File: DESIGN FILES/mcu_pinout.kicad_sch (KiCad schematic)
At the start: 16 parts, among them U1 MIMXRT1064CVL5B

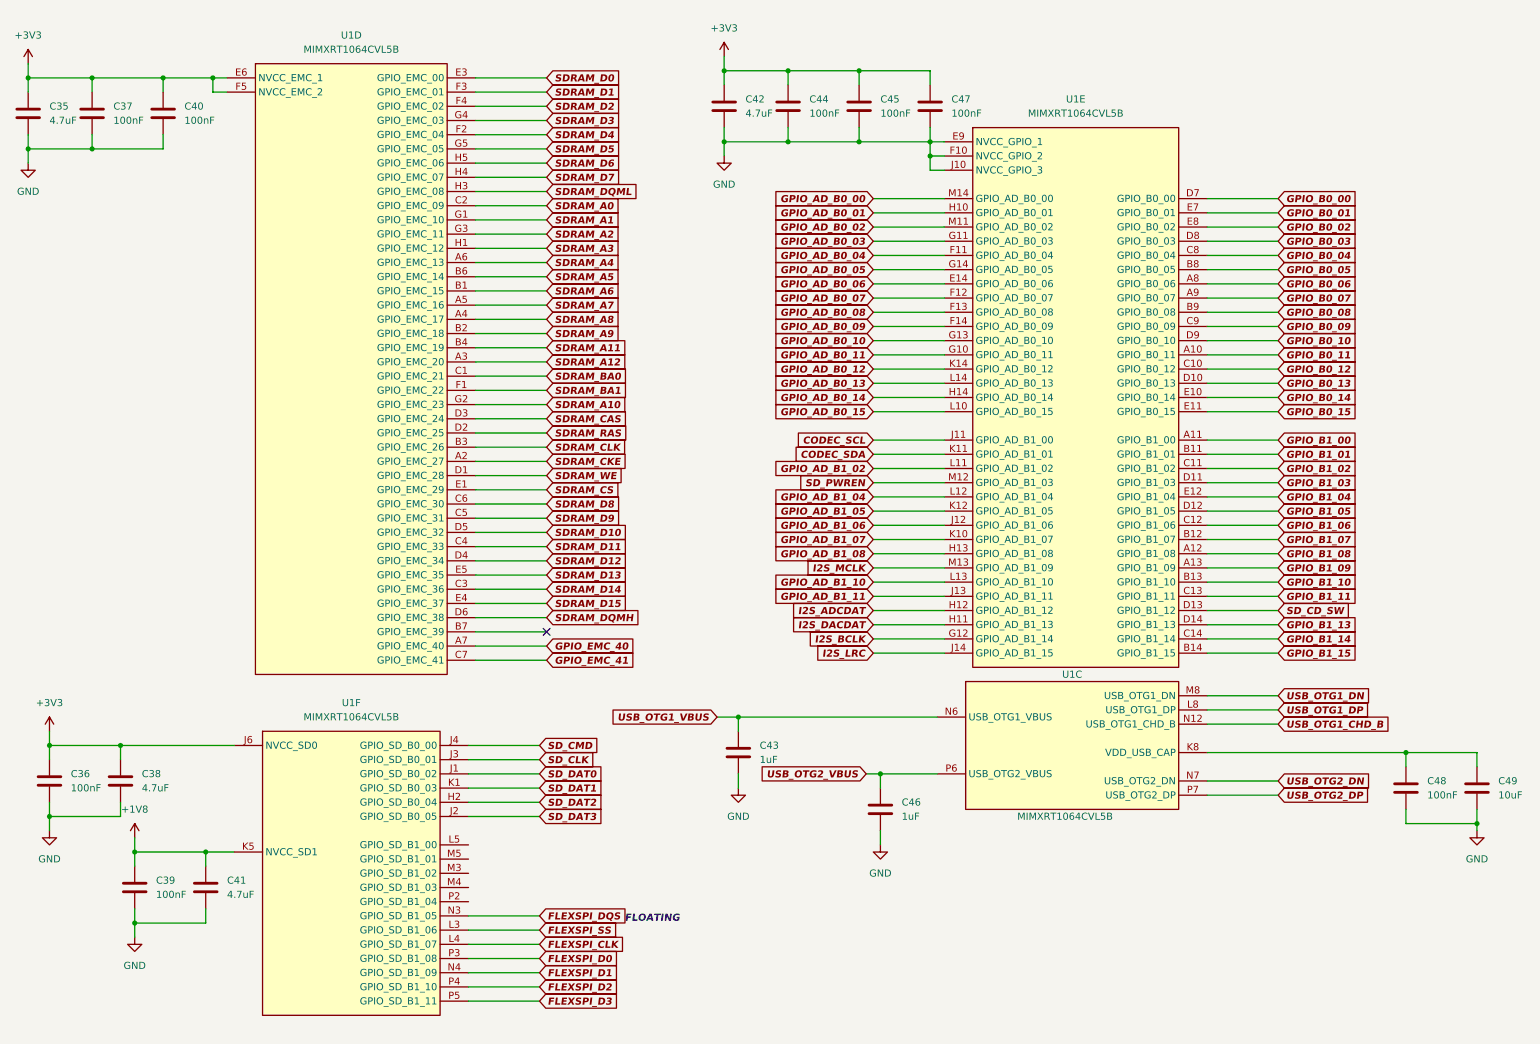
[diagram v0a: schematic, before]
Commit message: Refactoring schematic
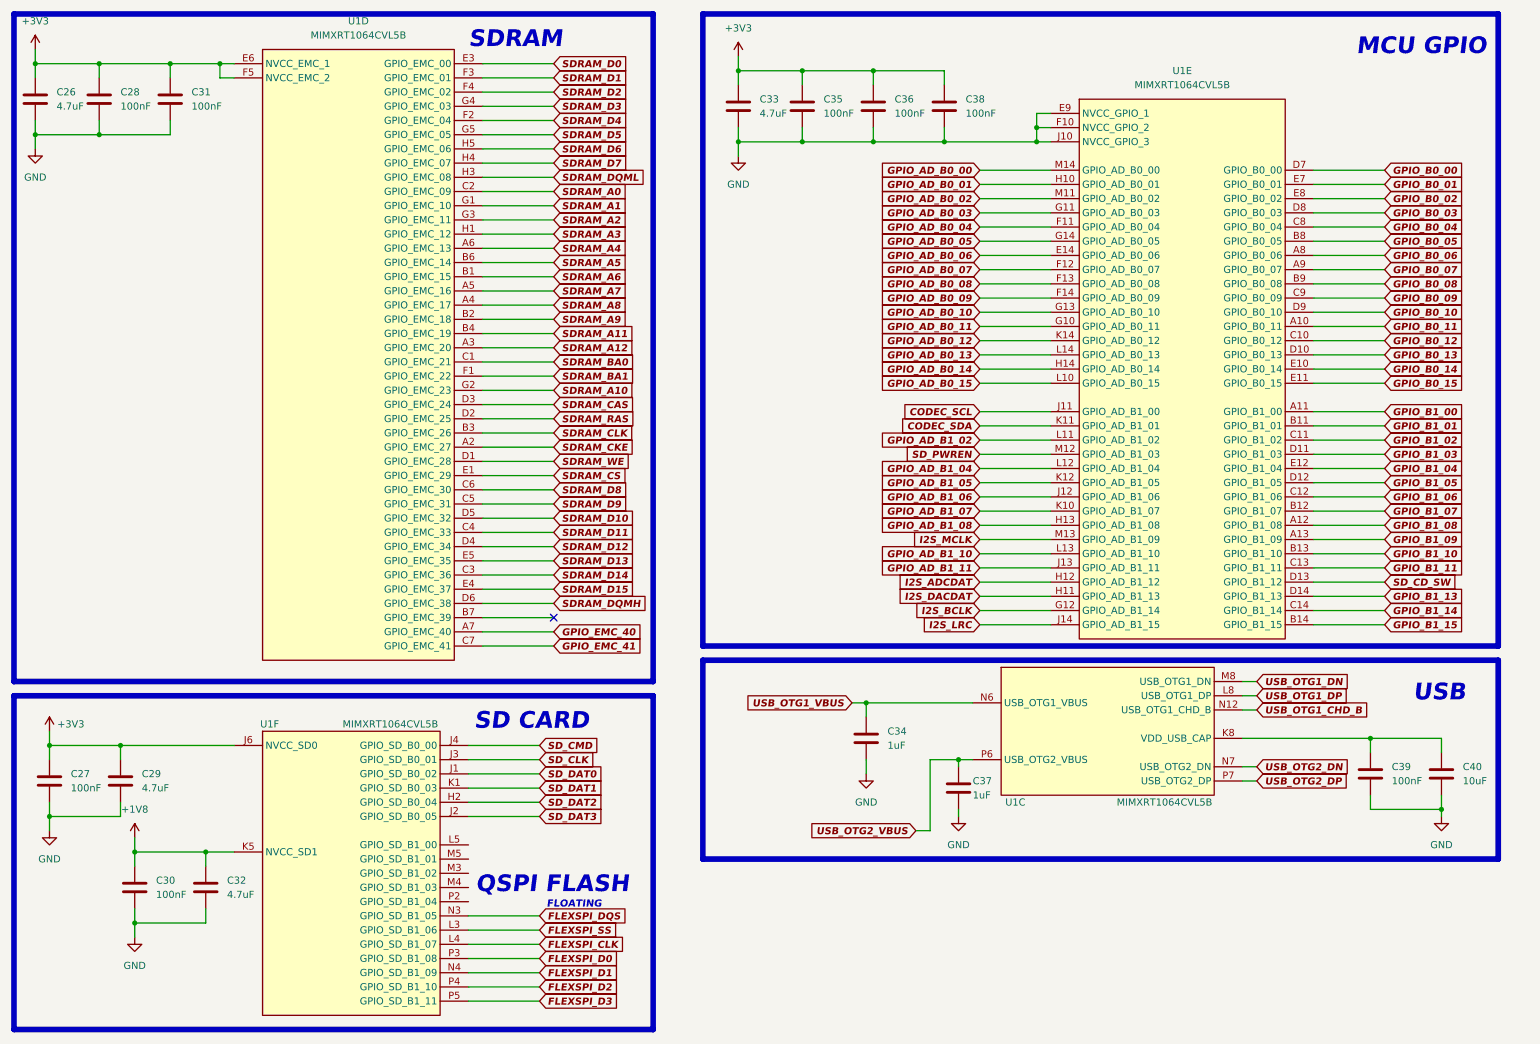
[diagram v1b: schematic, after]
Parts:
- renumbered C35 to C26, C36 to C27, C37 to C28, C38 to C29, C39 to C30, C40 to C31, C41 to C32, C42 to C33, C43 to C34, C44 to C35, C45 to C36, C46 to C37, C47 to C38, C48 to C39, C49 to C40
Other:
- note added: "MCU GPIO"
- note added: "QSPI FLASH"
- note added: "SD CARD"
- note added: "SDRAM"
- note added: "USB"
- moved on the sheet: C26, C28, C31, C33, C34, C35, C36, C37, C38, C39, C40, U1C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
